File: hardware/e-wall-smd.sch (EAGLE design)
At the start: 67 parts, among them IC1 74HCT595D, IC2 74HCT595D, IC3 74HCT595D, IC4 74HCT595D, Q1 2N7002P, Q10 2N7002P, Q11 2N7002P, Q12 2N7002P, Q13 2N7002P, Q14 2N7002P, Q15 2N7002P, Q16 2N7002P, Q17 2N7002P, Q18 2N7002P, Q19 2N7002P, Q2 2N7002P, Q20 2N7002P, Q21 2N7002P, Q22 2N7002P, Q23 2N7002P, Q24 2N7002P, Q25 IRF8313P, Q26 IRF8313P, Q27 IRF8313P, Q28 IRF8313P, Q3 2N7002P, Q4 2N7002P, Q5 2N7002P, Q6 2N7002P, Q7 2N7002P, Q8 2N7002P, Q9 2N7002P, T1 BC547, T2 BC557, T3 BC547

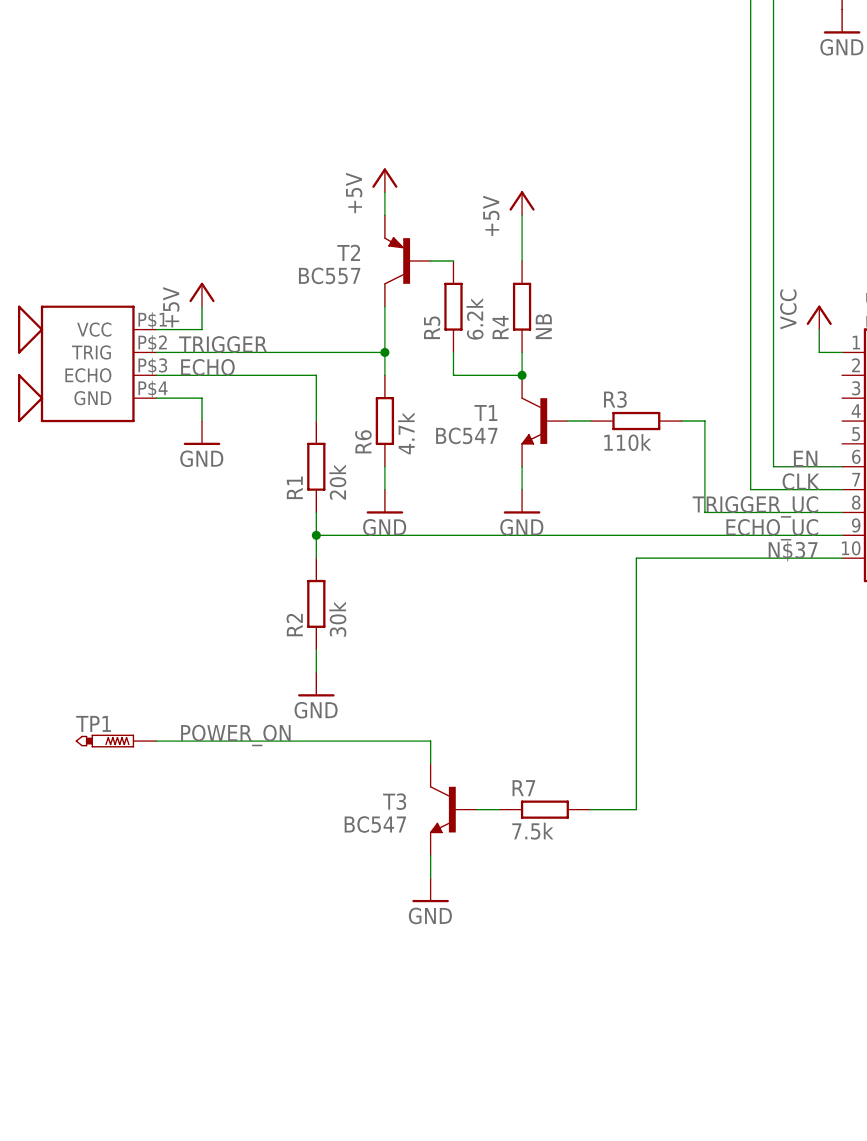
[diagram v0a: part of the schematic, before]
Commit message: Pegelwandler mit FET
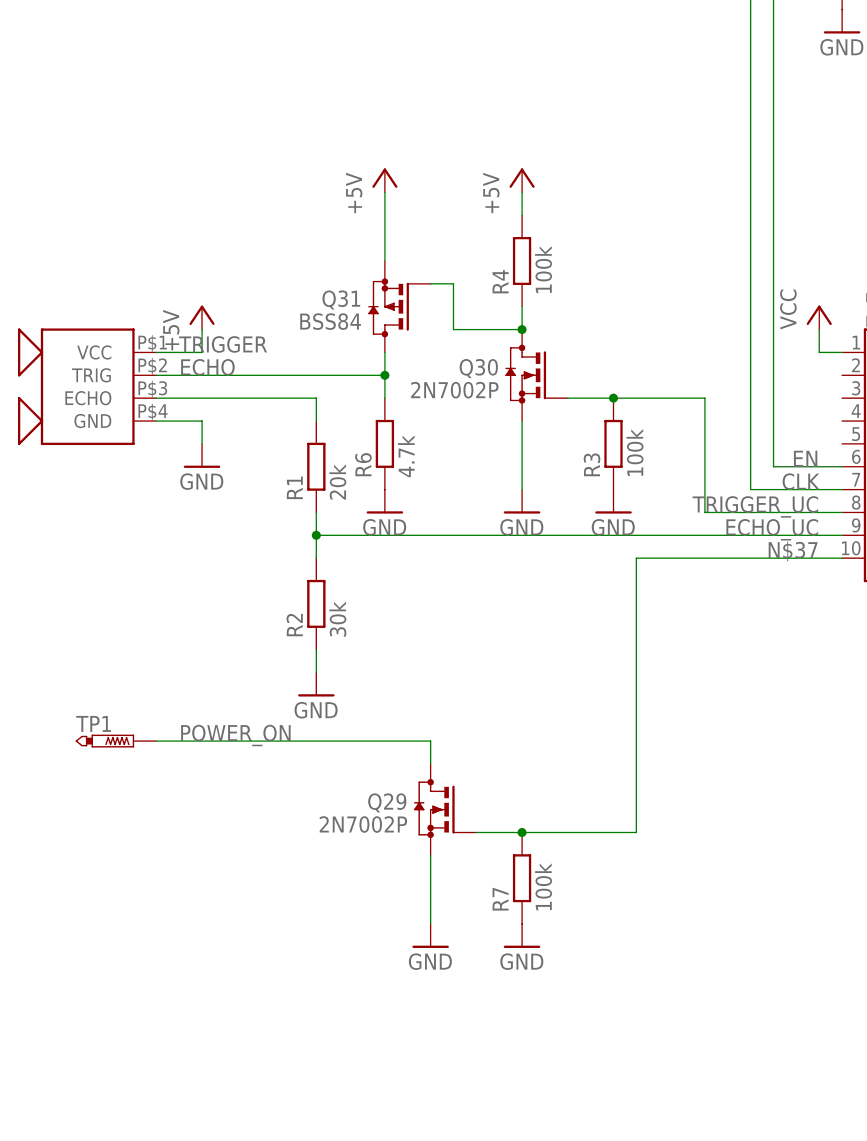
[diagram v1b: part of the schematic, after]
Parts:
- removed R5: 6.2k, resistor:R-EU_R1206
- removed T1, T3: BC547, transistor:-NPN-SOT23-EBC
- removed T2: BC557, transistor:-PNP-SOT23-BCE
- added Q29, Q30: 2N7002P, transistor-small-signal:BSS123
- added Q31: BSS84, transistor-small-signal:BSS84
- R3: value 110k -> 100k
- R4: value NB -> 100k
- R7: value 7.5k -> 100k
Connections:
- removed net CP: IC1A.G, IC1P.GND, IC2A.G, IC2P.GND, IC3A.G, IC3P.GND, IC4A.G, IC4P.GND, Q1.S, Q10.S, Q11.S, Q12.S, Q13.S, Q14.S, Q15.S, Q16.S, Q17.S, Q18.S, Q19.S, Q2.S, Q20.S, Q21.S, Q22.S, Q23.S, Q24.S, Q25A.S, Q25B.S, Q26A.S, Q26B.S, Q27A.S, Q27B.S, Q28A.S, Q28B.S, Q3.S, Q4.S, Q5.S, Q6.S, Q7.S, Q8.S, Q9.S, R2.1, R6.1, R9.1, T1.E, T3.E, TP4.TP, U$1.20, U$2.GND
- removed net N$33: R3.1, T1.B
- removed net N$35: R5.2, T2.B
- removed net N$36: R7.1, T3.B
- new net GND: IC1A.G, IC1P.GND, IC2A.G, IC2P.GND, IC3A.G, IC3P.GND, IC4A.G, IC4P.GND, Q1.S, Q10.S, Q11.S, Q12.S, Q13.S, Q14.S, Q15.S, Q16.S, Q17.S, Q18.S, Q19.S, Q2.S, Q20.S, Q21.S, Q22.S, Q23.S, Q24.S, Q25A.S, Q25B.S, Q26A.S, Q26B.S, Q27A.S, Q27B.S, Q28A.S, Q28B.S, Q29.S, Q3.S, Q30.S, Q4.S, Q5.S, Q6.S, Q7.S, Q8.S, Q9.S, R2.1, R3.1, R6.1, R7.1, R9.1, TP4.TP, U$1.20, U$2.GND
- net +5V: now also Q31.S; no longer T2.E
- net N$34: now also Q30.D, Q31.G; no longer R5.1, T1.C
- net N$37: now also Q29.G
- net POWER_ON: now also Q29.D; no longer T3.C
- net TRIGGER: now also Q31.D; no longer T2.C
- net TRIGGER_UC: now also Q30.G
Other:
- moved on the sheet: R3, R4, R6, R7
